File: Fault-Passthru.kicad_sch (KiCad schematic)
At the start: 12 parts, among them Q12 SI2347DS-T1-GE3, Q13 SI2318CDS-T1-GE3

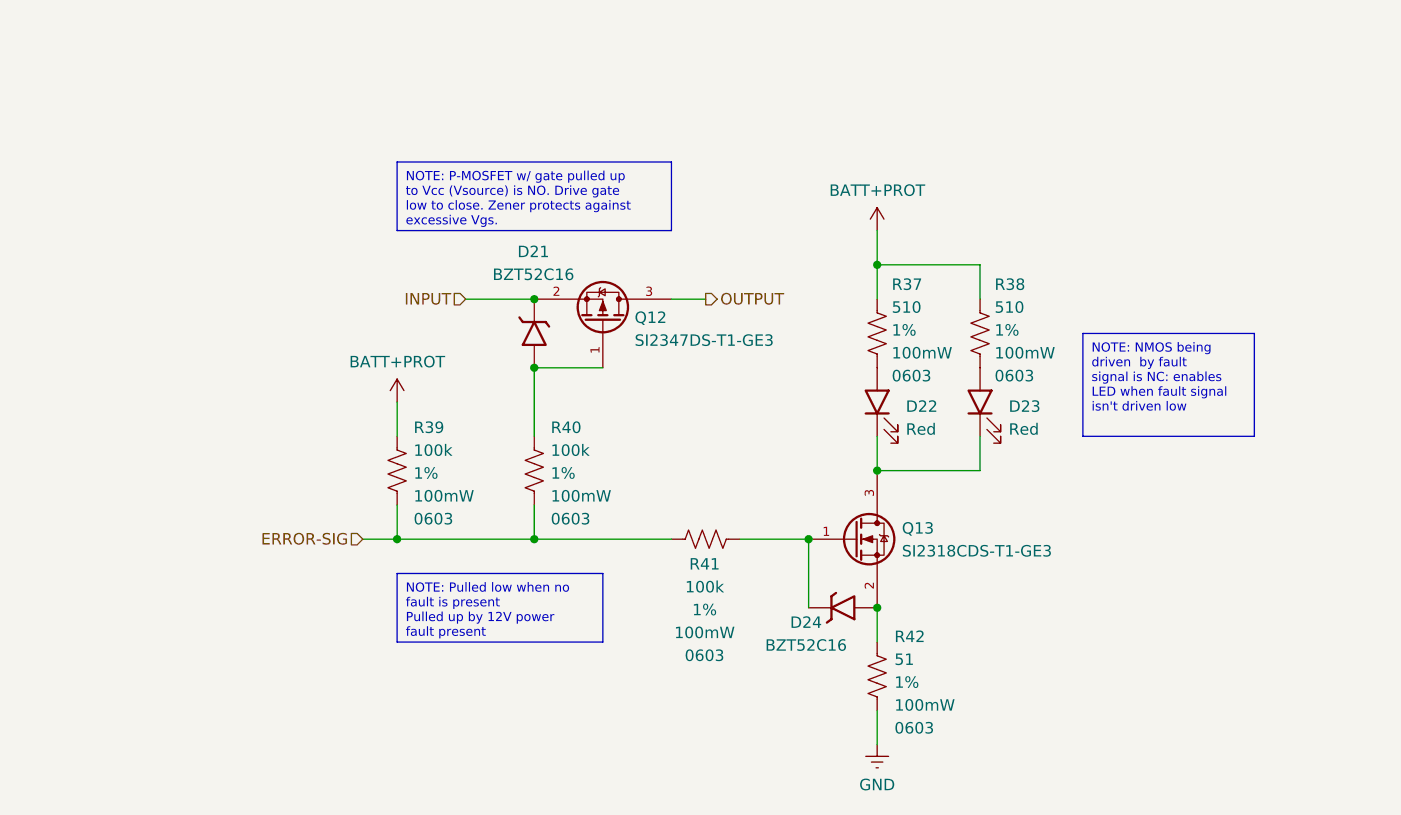
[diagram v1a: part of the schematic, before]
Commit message: schematic updated to V2 extra crispy
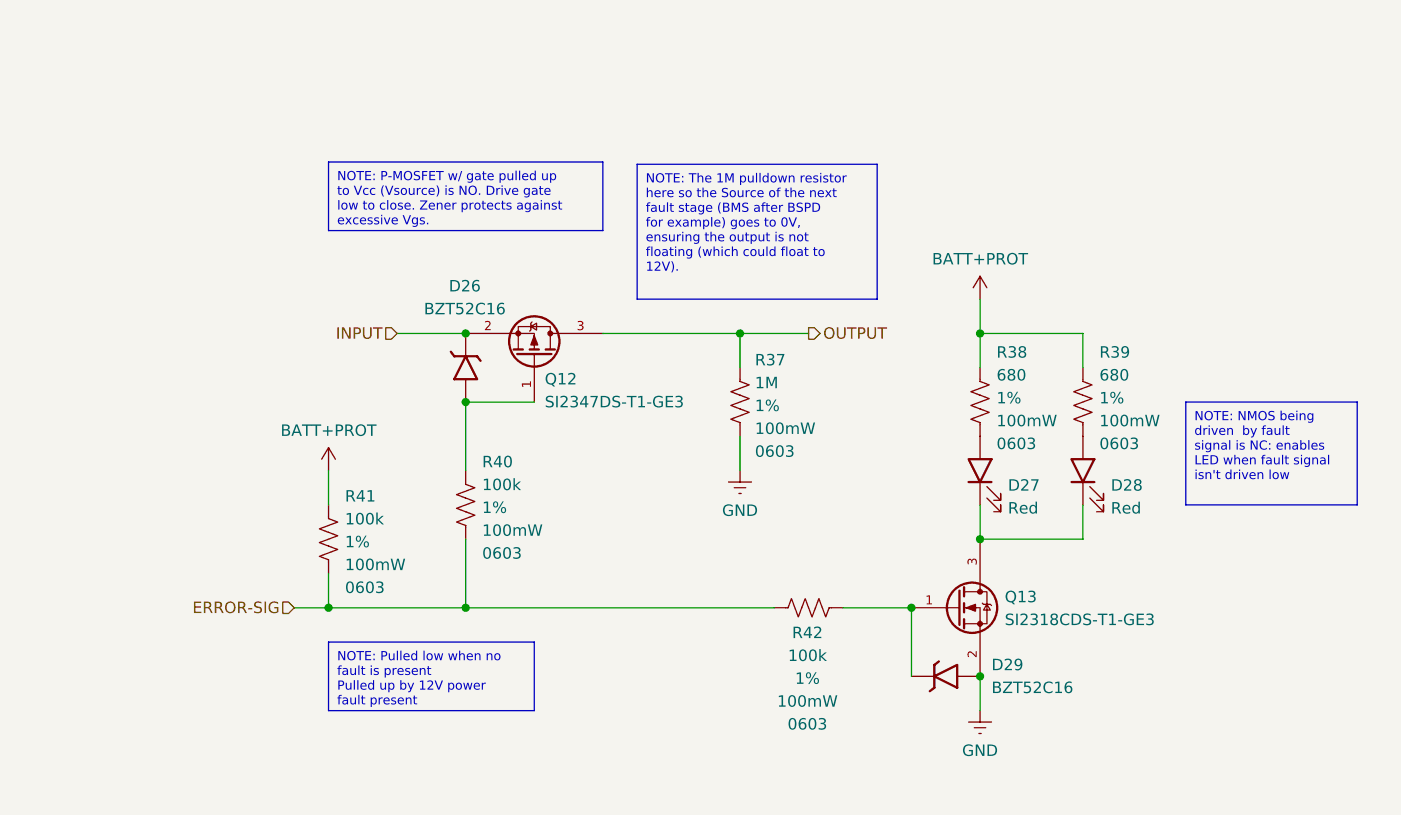
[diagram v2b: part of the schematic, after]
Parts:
- removed D22, D23: Red, LED_SMD:LED_0805_2012Metric, symbol -Diodes-LED:NCD0805R1
- removed R37, R38: 510, Resistor_SMD:R_0603_1608Metric_Pad0.98x0.95mm_HandSolder, symbol -R-SMD-0603:R-0603-510-1%-100mW-100PPM
- removed R42: 51, Resistor_SMD:R_0603_1608Metric_Pad0.98x0.95mm_HandSolder, symbol -R-SMD-0603:R-0603-51-1%-100mW-100PPM
- added D27, D28: Red, LED_SMD:LED_0805_2012Metric, symbol -Diodes-LED:NCD0805R1
- added R37: 1M, Resistor_SMD:R_0603_1608Metric_Pad0.98x0.95mm_HandSolder, symbol -R-SMD-0603:R-0603-1M-1%-100mW-100PPM
- added R38, R39: 680, Resistor_SMD:R_0603_1608Metric_Pad0.98x0.95mm_HandSolder, symbol -R-SMD-0603:R-0603-680-1%-100mW-100PPM
- renumbered D21 to D26, D24 to D29, R39 to R41, R41 to R42
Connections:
- net BATT+PROT: now also R38.2, R39.2
- net GND: now also D29.2 (A), Q13.2 (S), R37.1
- net OUTPUT: now also R37.2
- net at Q13.3 (D): now also D27.1 (K), D28.1 (K)
- new net: D27.2 (A), R38.1
- new net: D28.2 (A), R39.1
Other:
- moved on the sheet: D26, D29, Q12, Q13, R40, R41, R42

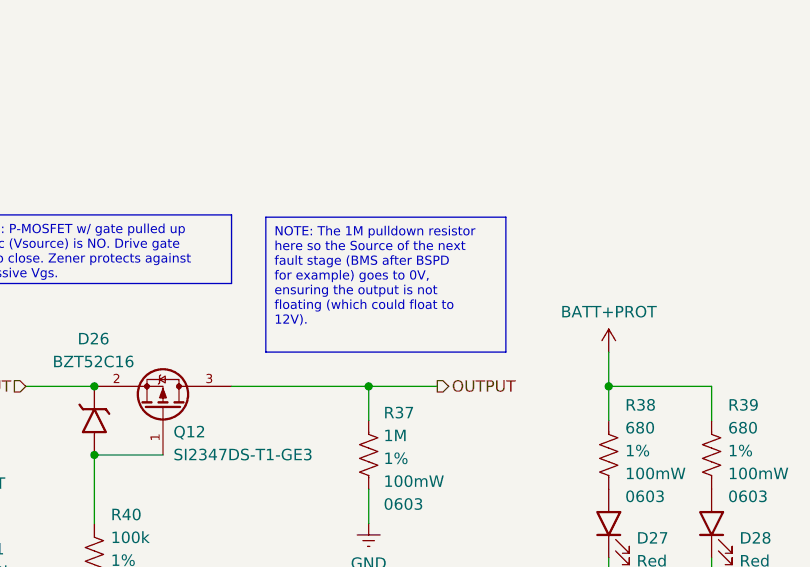
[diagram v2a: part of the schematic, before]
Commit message: layout done extra crispy v2
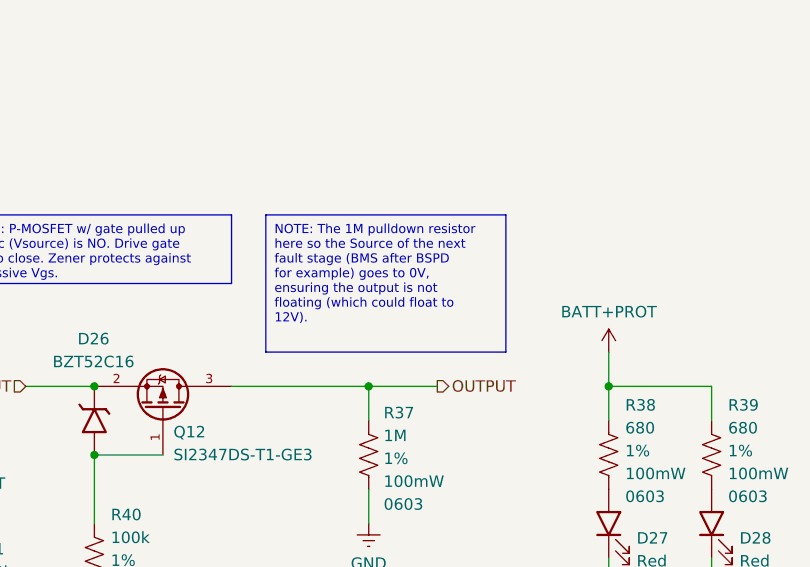
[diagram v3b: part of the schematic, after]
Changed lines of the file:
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@@
 	(text_box "NOTE: The 1M pulldown resistor here so the Source of the next fault stage (BMS after BSPD for example) goes to 0V, ensuring the output is not floating (which could float to 12V)."
 		(exclude_from_sim no)
-		(at 194.31 118.3606 0)
-		(size 26.67 14.9894)
+		(at 194.31 118.11 0)
+		(size 26.67 15.24)
 		(margins 0.9525 0.9525 0.9525 0.9525)
 		(stroke
